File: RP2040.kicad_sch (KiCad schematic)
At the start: 28 parts, among them J1 USB_B_Micro, J2 Conn_01x02, J3 RP2040_SWD, U1 RP2040, U2 AMS1117-3.3, U3 W25Q128JVS, Y1 X322512MSB4SI

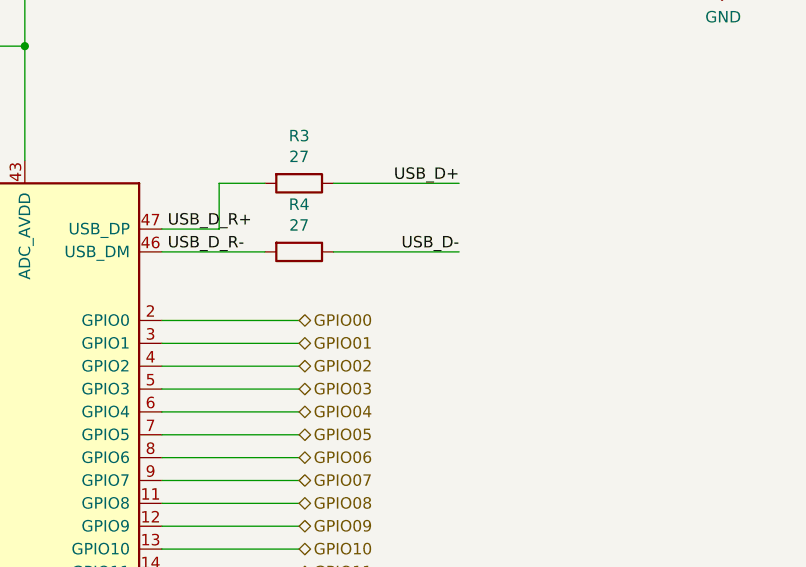
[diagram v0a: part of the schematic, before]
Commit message: More layout
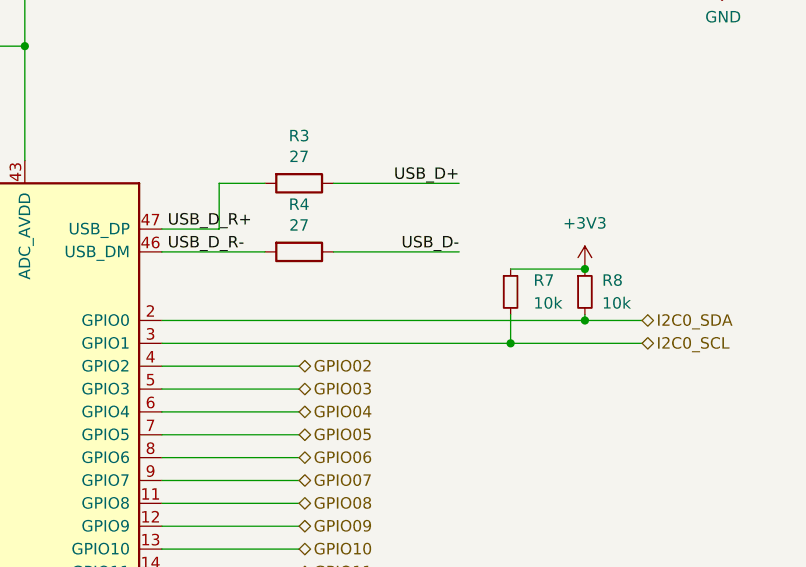
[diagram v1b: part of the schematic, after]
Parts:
- added R7, R8: 10k, Custom_Footprints:Perfect_0402, symbol Device:R_Small
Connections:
- net +3V3: now also R7.1, R8.1
- net GPIO00 renamed I2C0_SDA
- net I2C0_SDA: now also R8.2
- net GPIO01 renamed I2C0_SCL
- net I2C0_SCL: now also R7.2
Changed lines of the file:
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@@
   (junction (at 39.37 111.125) (diameter 0) (color 0 0 0 0)
   )
+  (junction (at 257.175 70.485) (diameter 0) (color 0 0 0 0)
+  )
   (junction (at 249.555 19.685) (diameter 0) (color 0 0 0 0)
   )
@@
   (junction (at 158.115 19.685) (diameter 0) (color 0 0 0 0)
   )
+  (junction (at 257.175 64.77) (diameter 0) (color 0 0 0 0)
+  )
   (junction (at 177.165 40.005) (diameter 0) (color 0 0 0 0)
   )
@@
   )
   (junction (at 36.83 24.13) (diameter 0) (color 0 0 0 0)
+  )
+  (junction (at 248.92 73.025) (diameter 0) (color 0 0 0 0)
   )
   (junction (at 74.295 60.96) (diameter 0) (color 0 0 0 0)
@@
   (no_connect (at 97.79 116.84))
   (no_connect (at 29.21 34.29))
+  (wire (pts (xy 257.175 70.485) (xy 257.175 69.85))
+    (stroke (width 0) (type default))
+  )
   (wire (pts (xy 139.065 20.955) (xy 139.065 19.685))
     (stroke (width 0) (type default))
@@
     (stroke (width 0) (type default))
   )
+  (wire (pts (xy 257.175 70.485) (xy 263.525 70.485))
+    (stroke (width 0) (type default))
+  )
   (polyline (pts (xy 13.97 106.045) (xy 13.97 130.175))
     (stroke (width 0) (type default))
   )
+  (wire (pts (xy 210.185 70.485) (xy 257.175 70.485))
+    (stroke (width 0) (type default))
+  )
   (polyline (pts (xy 74.93 106.045) (xy 101.6 106.045))
     (stroke (width 0) (type default))
@@
     (stroke (width 0) (type default))
   )
-  (wire (pts (xy 210.185 73.025) (xy 225.425 73.025))
-    (stroke (width 0) (type default))
-  )
   (wire (pts (xy 132.715 83.185) (xy 146.685 83.185))
     (stroke (width 0) (type default))
@@
     (stroke (width 0) (type default))
   )
+  (wire (pts (xy 210.185 73.025) (xy 248.92 73.025))
+    (stroke (width 0) (type default))
+  )
   (wire (pts (xy 210.185 108.585) (xy 225.425 108.585))
     (stroke (width 0) (type default))
@@
     (stroke (width 0) (type default))
   )
-  (wire (pts (xy 210.185 70.485) (xy 225.425 70.485))
-    (stroke (width 0) (type default))
-  )
   (wire (pts (xy 210.185 78.105) (xy 225.425 78.105))
     (stroke (width 0) (type default))
@@
     (stroke (width 0) (type default))
   )
+  (wire (pts (xy 248.92 73.025) (xy 248.92 69.85))
+    (stroke (width 0) (type default))
+  )
   (wire (pts (xy 210.185 62.865) (xy 221.615 62.865))
     (stroke (width 0) (type default))
@@
   )
   (wire (pts (xy 158.115 18.415) (xy 158.115 19.685))
+    (stroke (width 0) (type default))
+  )
+  (wire (pts (xy 248.92 64.77) (xy 257.175 64.77))
+    (stroke (width 0) (type default))
+  )
+  (wire (pts (xy 248.92 73.025) (xy 263.525 73.025))
     (stroke (width 0) (type default))
   )
@@
     (effects (font (size 1.27 1.27)) (justify left))
   )
-  (hierarchical_label "GPIO00" (shape bidirectional) (at 225.425 70.485 0) (fields_autoplaced)
-    (effects (font (size 1.27 1.27)) (justify left))
-  )
   (hierarchical_label "GPIO25" (shape bidirectional) (at 225.425 133.985 0) (fields_autoplaced)
     (effects (font (size 1.27 1.27)) (justify left))
@@
     (effects (font (size 1.27 1.27)) (justify left))
   )
-  (hierarchical_label "GPIO01" (shape bidirectional) (at 225.425 73.025 0) (fields_autoplaced)
-    (effects (font (size 1.27 1.27)) (justify left))
-  )
   (hierarchical_label "GPIO02" (shape bidirectional) (at 225.425 75.565 0) (fields_autoplaced)
     (effects (font (size 1.27 1.27)) (justify left))
@@
     (effects (font (size 1.27 1.27)) (justify left))
   )
+  (hierarchical_label "I2C0_SDA" (shape bidirectional) (at 263.525 70.485 0) (fields_autoplaced)
+    (effects (font (size 1.27 1.27)) (justify left))
+  )
   (hierarchical_label "GPIO23" (shape bidirectional) (at 225.425 128.905 0) (fields_autoplaced)
     (effects (font (size 1.27 1.27)) (justify left))
@@
   )
   (hierarchical_label "GPIO07" (shape bidirectional) (at 225.425 88.265 0) (fields_autoplaced)
+    (effects (font (size 1.27 1.27)) (justify left))
+  )
+  (hierarchical_label "I2C0_SCL" (shape bidirectional) (at 263.525 73.025 0) (fields_autoplaced)
     (effects (font (size 1.27 1.27)) (justify left))
   )
@@
         (path "/e63e39d7-6ac0-4ffd-8aa3-1841a4541b55/99e5628a-8c61-4f9d-aa6e-5b585271b505"
           (reference "J1") (unit 1)
+        )
+      )
+    )
+  )
+  (symbol (lib_id "Device:R_Small") (at 257.175 67.31 0) (unit 1)
+    (in_bom yes) (on_board yes) (dnp no) (fields_autoplaced)
+    (property "Reference" "R8" (at 259.08 66.04 0)
+      (effects (font (size 1.27 1.27)) (justify left))
+    )
+    (property "Value" "10k" (at 259.08 68.58 0)
+      (effects (font (size 1.27 1.27)) (justify left))
+    )
+    (property "Footprint" "Custom_Footprints:Perfect_0402" (at 257.175 67.31 0)
+      (effects (font (size 1.27 1.27)) hide)
+    )
+    (property "Datasheet" "~" (at 257.175 67.31 0)
+      (effects (font (size 1.27 1.27)) hide)
+    )
+    (property "MPN - JLCPCB" "C25744" (at 257.175 67.31 0)
+      (effects (font (size 1.27 1.27)) hide)
+    )
+    (pin "1")
+    (pin "2")
+    (instances
+      (project "RP2040-Radio-Panel"
+        (path "/e63e39d7-6ac0-4ffd-8aa3-1841a4541b55/99e5628a-8c61-4f9d-aa6e-5b585271b505"
+          (reference "R8") (unit 1)
         )
       )
@@
         )
       )
+    )
+  )
+  (symbol (lib_name "+3V3_1") (lib_id "power:+3V3") (at 257.175 64.77 0) (unit 1)
+    (in_bom yes) (on_board yes) (dnp no) (fields_autoplaced)
+    (property "Reference" "#PWR026" (at 257.175 68.58 0)
+      (effects (font (size 1.27 1.27)) hide)
+    )
+    (property "Value" "+3V3" (at 257.175 59.69 0)
+      (effects (font (size 1.27 1.27)))
+    )
+    (property "Footprint" "" (at 257.175 64.77 0)
+      (effects (font (size 1.27 1.27)) hide)
+    )
+    (property "Datasheet" "" (at 257.175 64.77 0)
+      (effects (font (size 1.27 1.27)) hide)
+    )
+    (pin "1")
+    (instances
+      (project "RP2040-Radio-Panel"
+        (path "/e63e39d7-6ac0-4ffd-8aa3-1841a4541b55/99e5628a-8c61-4f9d-aa6e-5b585271b505"
+          (reference "#PWR026") (unit 1)
+        )
+      )
+    )
+  )
+  (symbol (lib_id "Device:R_Small") (at 248.92 67.31 0) (unit 1)
+    (in_bom yes) (on_board yes) (dnp no) (fields_autoplaced)
+    (property "Reference" "R7" (at 251.46 66.04 0)
+      (effects (font (size 1.27 1.27)) (justify left))
+    )
+    (property "Value" "10k" (at 251.46 68.58 0)
+      (effects (font (size 1.27 1.27)) (justify left))
+    )
+    (property "Footprint" "Custom_Footprints:Perfect_0402" (at 248.92 67.31 0)
+      (effects (font (size 1.27 1.27)) hide)
+    )
+    (property "Datasheet" "~" (at 248.92 67.31 0)
+      (effects (font (size 1.27 1.27)) hide)
+    )
+    (property "MPN - JLCPCB" "C25744" (at 248.92 67.31 0)
+      (effects (font (size 1.27 1.27)) hide)
+    )
+    (pin "1")
+    (pin "2")
+    (instances
+      (project "RP2040-Radio-Panel"
+        (path "/e63e39d7-6ac0-4ffd-8aa3-1841a4541b55/99e5628a-8c61-4f9d-aa6e-5b585271b505"
+          (reference "R7") (unit 1)
+        )
+      )
